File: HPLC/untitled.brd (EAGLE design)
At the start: 84 x 125 mm, 18 parts, among them U2 AMS1117, U3 MAX232CSE, X1 MSTBA2, X2 MSTBA4, X3 C-GRID-02-70543, X4 MSTBA3

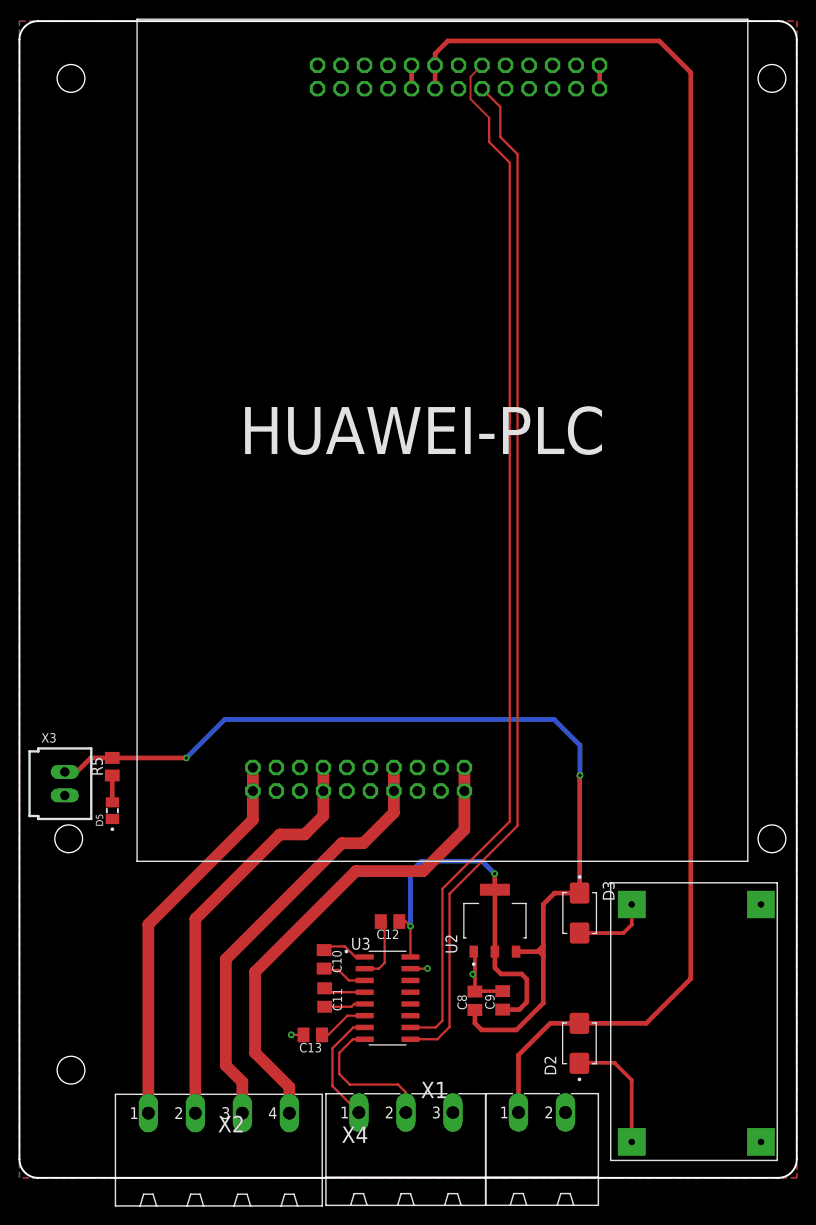
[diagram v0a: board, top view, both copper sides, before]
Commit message: revisi HPLC
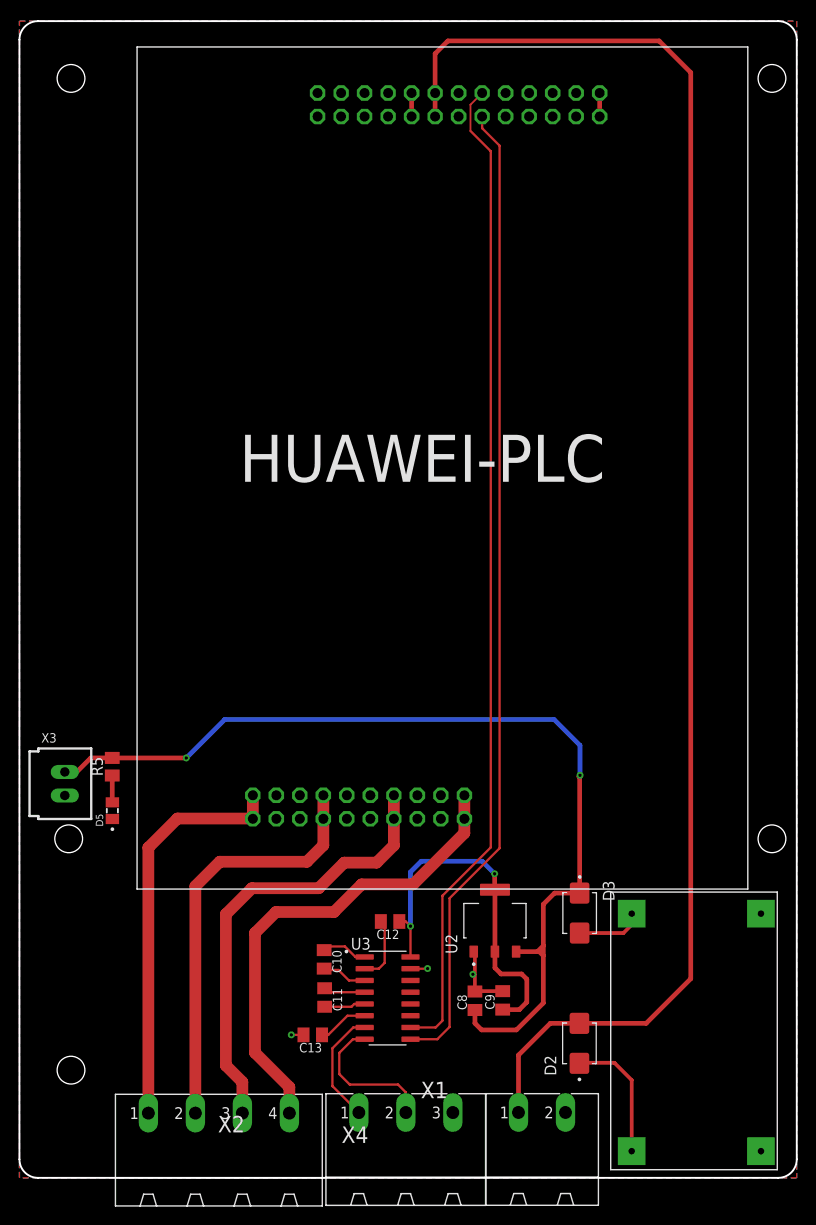
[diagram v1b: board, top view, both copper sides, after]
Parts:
- moved HUAWEI-PLC1 3.00 mm to (51.7, 122.2)
- moved MINI1 1.00 mm to (64.9, 2.88)
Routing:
- net TX_RS232: track 112.3 -> 107.6 mm
- net RX_RS232: track 110.8 -> 106.2 mm
- net 12V: track 159.6 -> 162.6 mm
- net PLC-C: track 47.0 -> 48.9 mm
- net PLC-A: track 42.0 -> 43.8 mm
- net N$9: track 8.20 -> 7.20 mm
- net N$7: track 13.1 -> 14.1 mm
- net PLC-B: track 44.6 -> 45.6 mm
